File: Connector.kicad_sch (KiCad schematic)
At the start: 3 parts, among them J7 Conn_02x10_Odd_Even

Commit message: Не битый репозиторий
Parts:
- J7: footprint Connector_PinSocket_2.54mm:PinSocket_2x10_P2.54mm_Vertical -> Connector_PinSocket_2.00mm:PinSocket_2x10_P2.00mm_Vertical
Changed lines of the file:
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@@
       (effects (font (size 1.27 1.27)) hide)
     )
-    (property "Footprint" "Connector_PinSocket_2.54mm:PinSocket_2x10_P2.54mm_Vertical" (at 156.21 83.82 0)
+    (property "Footprint" "Connector_PinSocket_2.00mm:PinSocket_2x10_P2.00mm_Vertical" (at 156.21 83.82 0)
       (effects (font (size 1.27 1.27)) hide)
     )

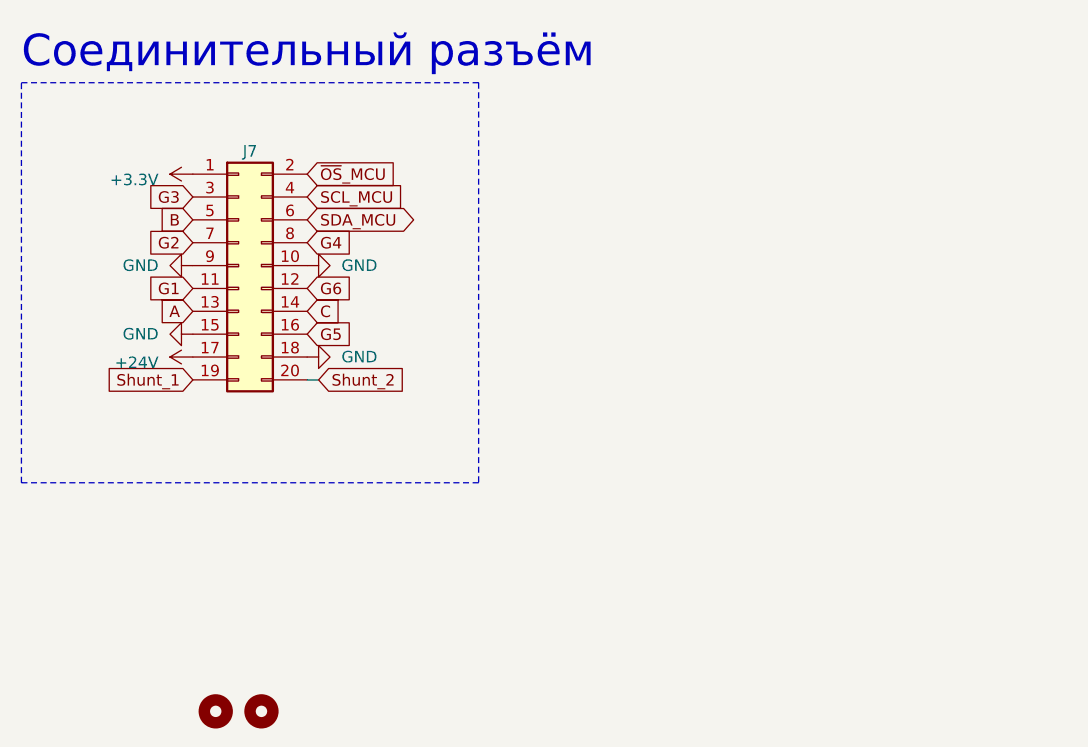
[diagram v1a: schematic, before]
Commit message: Первый вариант
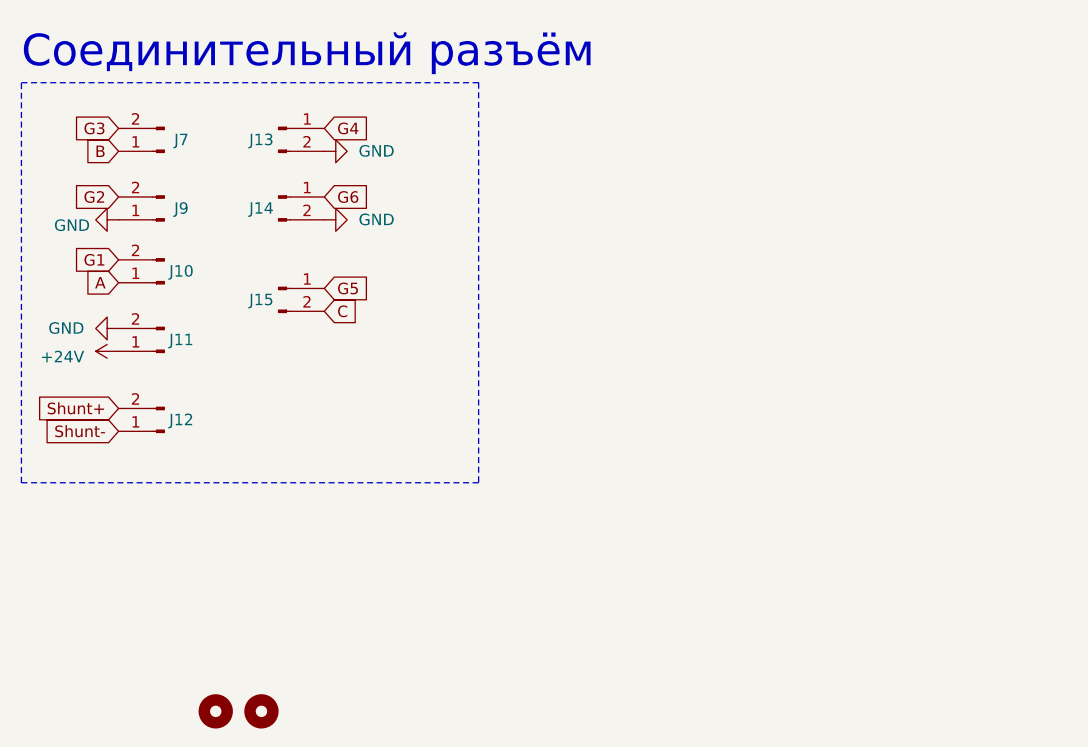
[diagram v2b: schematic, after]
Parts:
- removed J7: Conn_02x10_Odd_Even, Connector_PinSocket_2.00mm:PinSocket_2x10_P2.00mm_Vertical, symbol Connector_Generic:Conn_02x10_Odd_Even
- added J10, J11, J12, J13, J14, J15, J7, J9: Conn_01x02_Pin, Connector_PinHeader_2.54mm:PinHeader_1x02_P2.54mm_Vertical_SMD_Pin1Left, symbol Connector:Conn_01x02_Pin
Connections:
- net +24V: now also J11.1 (Pin_1)
- net A: now also J10.1 (Pin_1)
- net B: now also J7.1 (Pin_1)
- net C: now also J15.2 (Pin_2)
- net G1: now also J10.2 (Pin_2)
- net G2: now also J9.2 (Pin_2)
- net G3: now also J7.2 (Pin_2)
- net G4: now also J13.1 (Pin_1)
- net G5: now also J15.1 (Pin_1)
- net G6: now also J14.1 (Pin_1)
- net GND: now also J11.2 (Pin_2), J13.2 (Pin_2), J14.2 (Pin_2), J9.1 (Pin_1)
- new net Shunt+: J12.2 (Pin_2)
- new net Shunt-: J12.1 (Pin_1)
